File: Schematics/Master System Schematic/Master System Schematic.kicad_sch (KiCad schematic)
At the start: 53 parts, among them M1 Cooling Pump, M2 RadFan, M3 RadFan, SW1 GLVMS, SW2 Side BRB, SW3 Side BRB, SW4 Brake Over-Travel Switch, SW6 Cockpit BRB, SW7 TSMS, SW8 SW_SPST_Pressure, SW9 SW_SPST_Pressure, U2 RinehartPM100DX_MotorControll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, U3 Emrax 228MV Motor

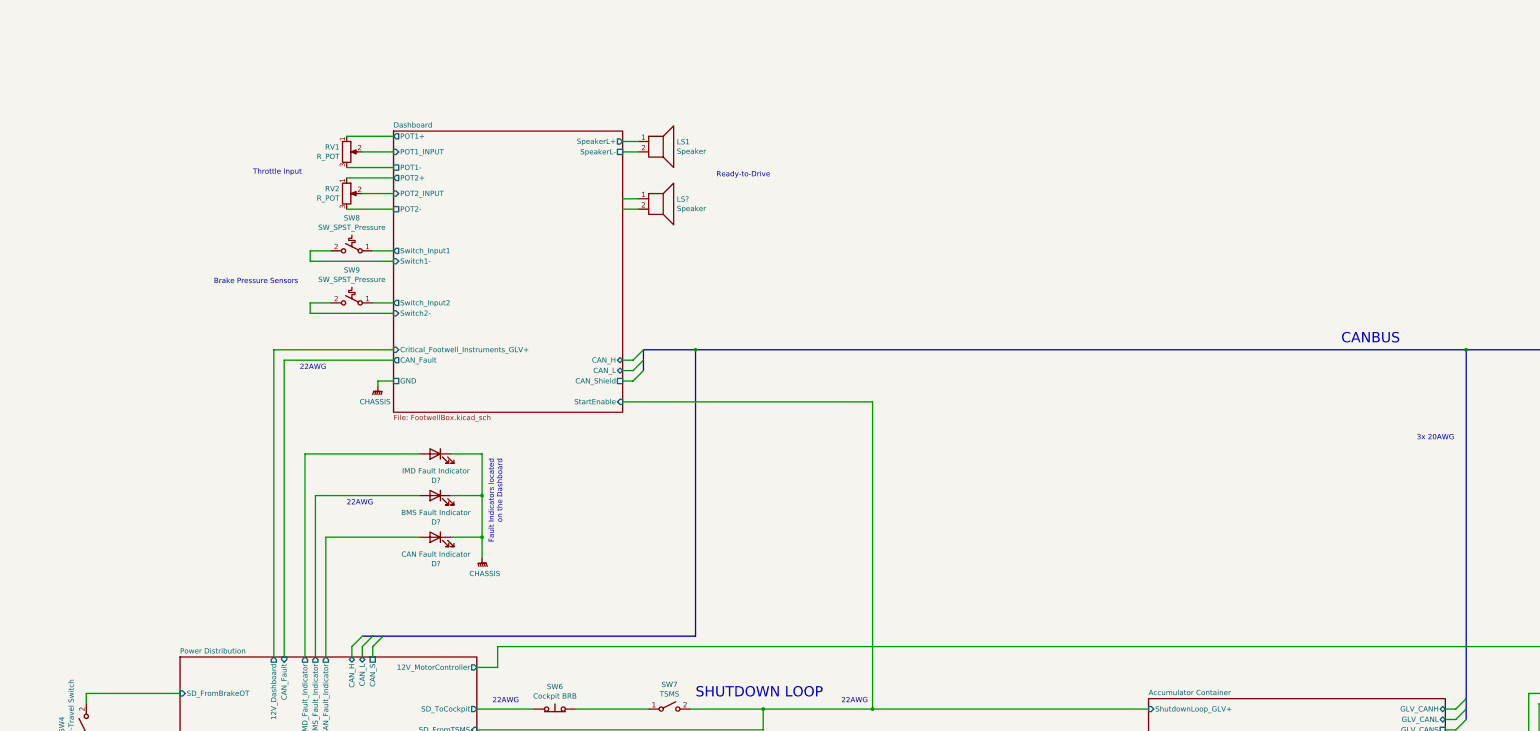
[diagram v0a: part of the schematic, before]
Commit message: Footwell updates
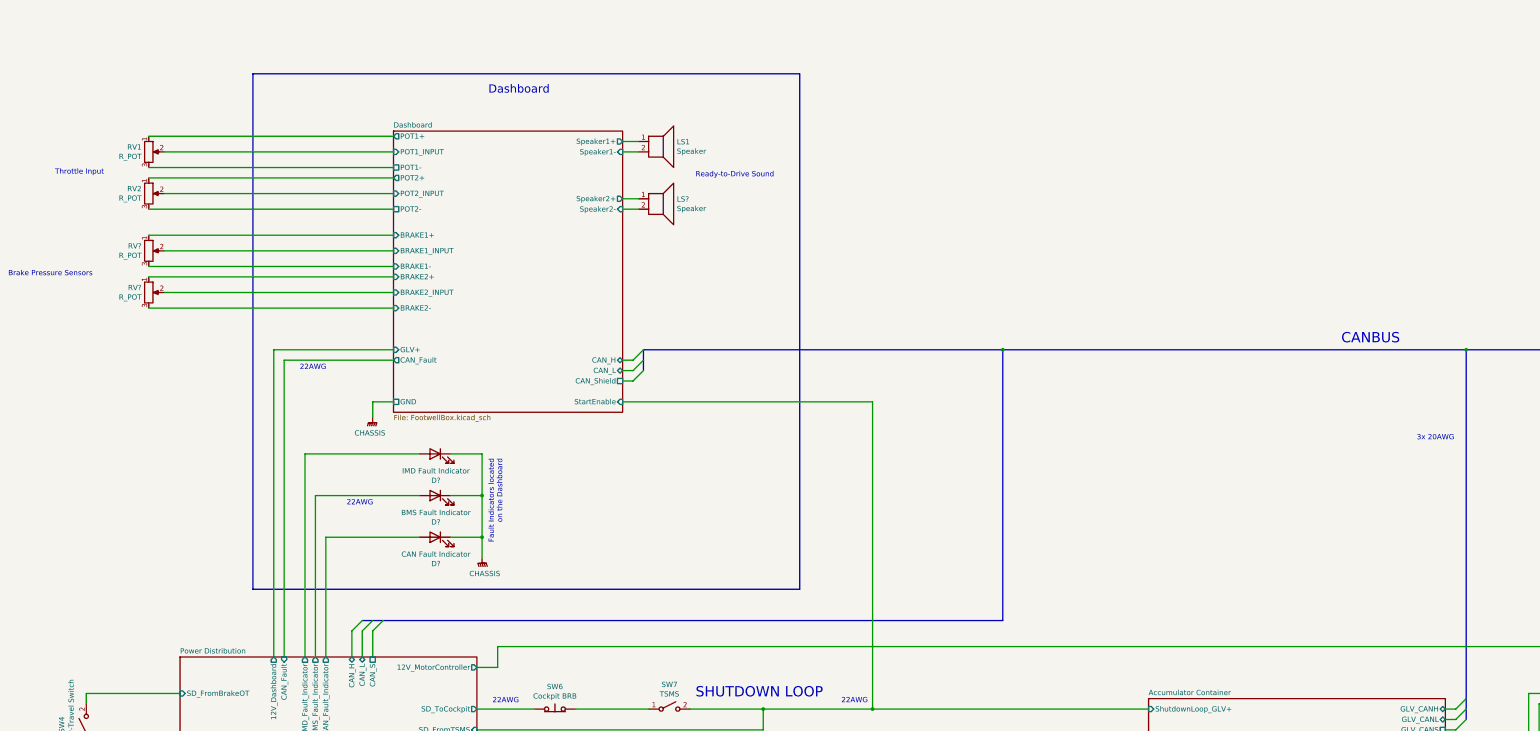
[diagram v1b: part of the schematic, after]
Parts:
- removed SW8, SW9: SW_SPST_Pressure, symbol Switch:SW_SPST_Temperature
- added RV? (x2): R_POT, symbol Device:R_POT
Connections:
- net at U3.~ (Resolver_IF): now also U2.~ (TS-)
- net Dashboard/Speaker2+: now reaches LS?.1
- net Dashboard/Speaker2-: now reaches LS?.2
- net Dashboard/SpeakerL+ renamed Dashboard/Speaker1+
- net Dashboard/SpeakerL- renamed Dashboard/Speaker1-
- new net: U2.~ (TS-), U3.~ (Resolver_IF) (x2)
- new net Dashboard/BRAKE1+: RV?.1
- new net Dashboard/BRAKE1-: RV?.3
- new net Dashboard/BRAKE1_INPUT: RV?.2
- new net Dashboard/BRAKE2+: RV?.1
- new net Dashboard/BRAKE2-: RV?.3
- new net Dashboard/BRAKE2_INPUT: RV?.2
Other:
- sheet Dashboard ports: added BRAKE1+, BRAKE1-, BRAKE1_INPUT, BRAKE2+, BRAKE2-, BRAKE2_INPUT, GLV+, Speaker1+, Speaker1-, Speaker2+, Speaker2-; removed Critical_Footwell_Instruments_GLV+, SpeakerL+, SpeakerL-, Switch1-, Switch2-, Switch_Input1, Switch_Input2
- note added: "Dashboard"
- note added: "Ready-to-Drive Sound"
- note removed: "Ready-to-Drive"
- moved on the sheet: RV1, RV2
